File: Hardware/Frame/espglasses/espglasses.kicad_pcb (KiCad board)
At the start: 2 copper layers, 170 x 45 mm, 13 parts, among them J1 BATTERY_1S, J2 OLED_SH1106_I2C, J3 TOUCH_INPUTS, J4 AUDIO_OUT_MONO, J5 UART_BOOT_DEBUG, J6 LED_STATUS, U1 ESP32_DEV_BOARD_PIN_BREAKOUT

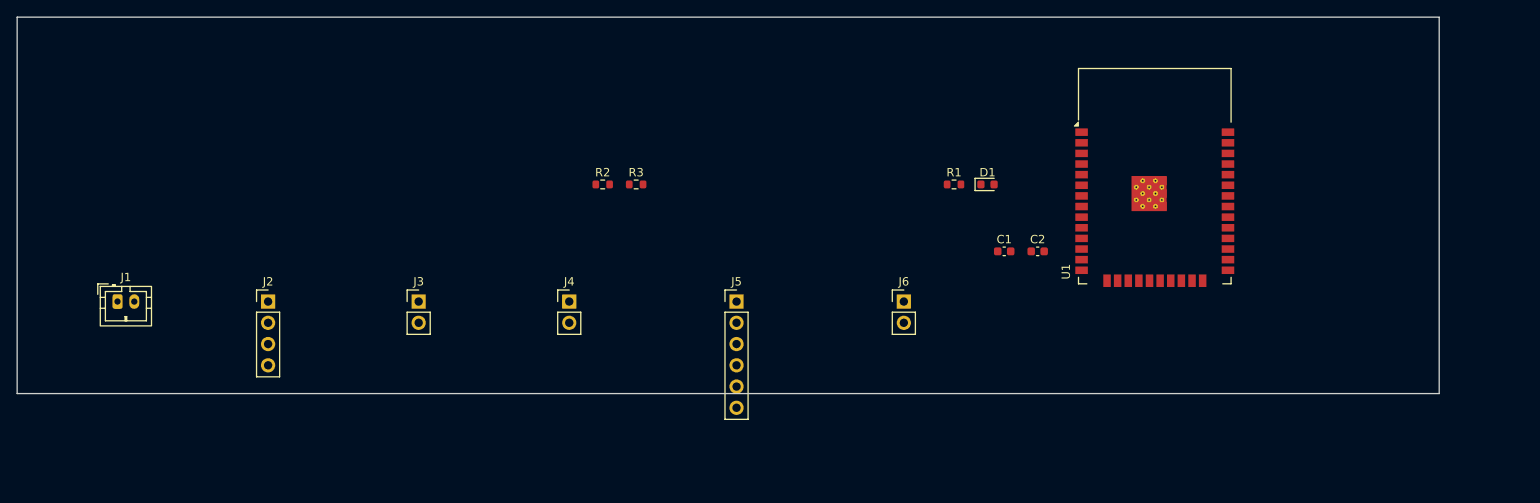
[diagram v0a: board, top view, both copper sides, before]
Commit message: kicad checkpoint 2
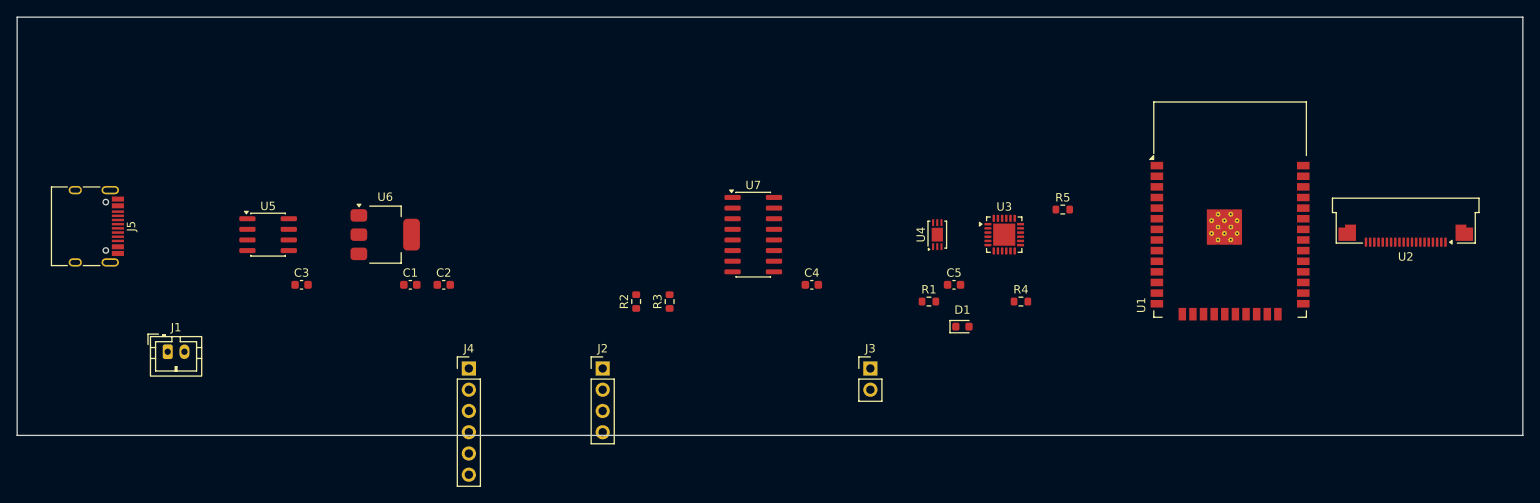
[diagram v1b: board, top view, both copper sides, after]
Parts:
- removed J6: LED_STATUS, PinHeader_1x02_P2.54mm_Vertical
- added C3: 10uF, C_0603_1608Metric, F.Cu at (34.0, 32.0)
- added C4: 100nF, C_0603_1608Metric, F.Cu at (95.0, 32.0)
- added C5: 100nF, C_0603_1608Metric, F.Cu at (112.0, 32.0)
- added R4: 10k, R_0603_1608Metric, F.Cu at (120.0, 34.0)
- added R5: 10k, R_0603_1608Metric, F.Cu at (125.0, 23.0)
- added U2: OV2640_CAMERA_IF, Amphenol_F32Q-1A7x1-11020_1x20-1MP_P0.5mm_Horizontal, F.Cu at (166.0, 24.0)
- added U3: MPU6050_CORE, QFN-24-1EP_4x4mm_P0.5mm_EP2.65x2.65mm, F.Cu at (118.0, 26.0)
- added U4: INMP441_CORE, DFN-6-1EP_3x2mm_P0.5mm_EP1.65x1.35mm, F.Cu at (110.0, 26.0)
- added U5: LIION_CHARGER_IC_CORE, SOIC-8_3.9x4.9mm_P1.27mm, F.Cu at (30.0, 26.0)
- added U6: REGULATOR_3V3_CORE, SOT-223-3_TabPin2, F.Cu at (44.0, 26.0)
- added U7: AUDIO_AMP_CORE, SOIC-16_3.9x9.9mm_P1.27mm, F.Cu at (88.0, 26.0)
- J2: value OLED_SH1106_I2C -> OLED_I2C_PANEL
- J3: value TOUCH_INPUTS -> SPEAKER_8OHM
- J4: value AUDIO_OUT_MONO -> UART_BOOT_DEBUG; footprint PinHeader_1x02_P2.54mm_Vertical -> PinHeader_1x06_P2.54mm_Vertical
- J5: value UART_BOOT_DEBUG -> USBC_POWER_IN; footprint PinHeader_1x06_P2.54mm_Vertical -> USB_C_Receptacle_HRO_TYPE-C-31-M-12
- U1: value ESP32_DEV_BOARD_PIN_BREAKOUT -> ESP32_WROVER_E_CORE
- moved J5 78.5 mm to (8.00, 25.0), turned to -90 degrees
- moved C1 71.1 mm to (47.0, 32.0)
- moved C2 71.1 mm to (51.0, 32.0)
- moved J3 54.6 mm to (102.0, 42.0)
- moved J2 40.8 mm to (70.0, 42.0)
- moved D1 17.3 mm to (113.0, 37.0)
- moved R2 14.6 mm to (74.0, 34.0), turned to 90 degrees
- moved R3 14.6 mm to (78.0, 34.0), turned to 90 degrees
- moved J4 14.4 mm to (54.0, 42.0)
- moved R1 14.3 mm to (109.0, 34.0)
- moved U1 9.85 mm to (145.0, 26.0)
- moved J1 8.49 mm to (18.0, 40.0)
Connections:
- C1 pad 1: +3V3_DIG -> (no net)
- C1 pad 2: GND -> (no net)
- C2 pad 1: +3V3_DIG -> (no net)
- C2 pad 2: GND -> (no net)
- D1 pad 1: GND -> (no net)
- D1 pad 2: LED_A -> (no net)
- J1 pad 1: VBAT_RAW -> (no net)
- J1 pad 2: GND -> (no net)
- J2 pad 1: +3V3_DIG -> (no net)
- J2 pad 2: GND -> (no net)
- J2 pad 3: I2C_SCL -> (no net)
- J2 pad 4: I2C_SDA -> (no net)
- J3 pad 1: TOUCH1_IN -> (no net)
- J3 pad 2: TOUCH2_IN -> (no net)
- J4 pad 1: DAC_SUM -> (no net)
- J4 pad 2: GND -> (no net)
- R1 pad 1: LED_STAT -> (no net)
- R1 pad 2: LED_A -> (no net)
- R2 pad 1: DAC_L_OUT -> (no net)
- R2 pad 2: DAC_SUM -> (no net)
- R3 pad 1: DAC_R_OUT -> (no net)
- R3 pad 2: DAC_SUM -> (no net)
- U1 pad 1: GND -> (no net)
- U1 pad 10: UART_TX_DBG -> (no net)
- U1 pad 12: UART_RX_DBG -> (no net)
- U1 pad 14: DAC_R_OUT -> (no net)
- U1 pad 16: DAC_L_OUT -> (no net)
- U1 pad 2: +3V3_DIG -> (no net)
- U1 pad 24: TOUCH2_IN -> (no net)
- U1 pad 26: TOUCH1_IN -> (no net)
- U1 pad 32: I2C_SCL -> (no net)
- U1 pad 34: I2C_SDA -> (no net)
- U1 pad 4: IO0 -> (no net)
- U1 pad 6: EN -> (no net)
- U1 pad 8: LED_STAT -> (no net)
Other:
- board size 170 x 45 mm -> 180 x 50 mm
